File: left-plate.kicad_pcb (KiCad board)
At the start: 2 copper layers, 155.6 x 97.3 mm, 26 parts

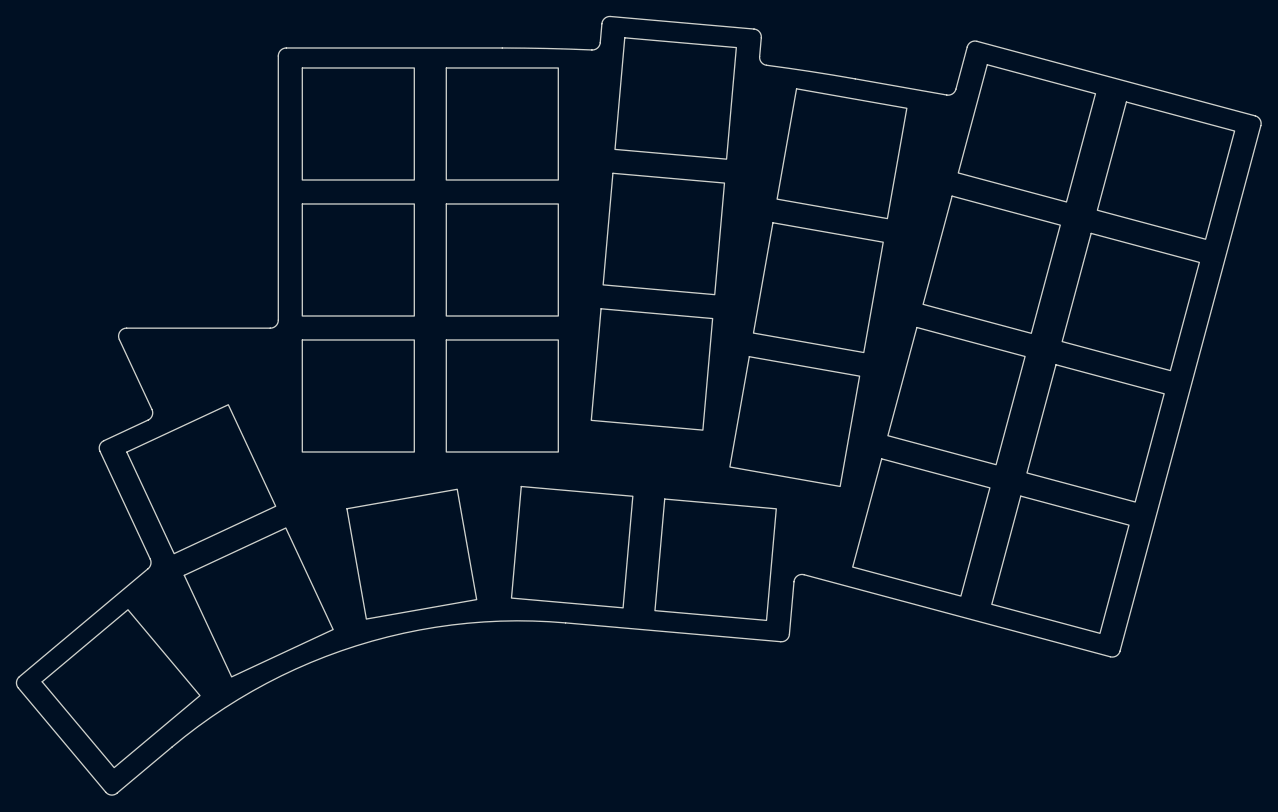
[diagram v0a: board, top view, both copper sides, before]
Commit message: update plates
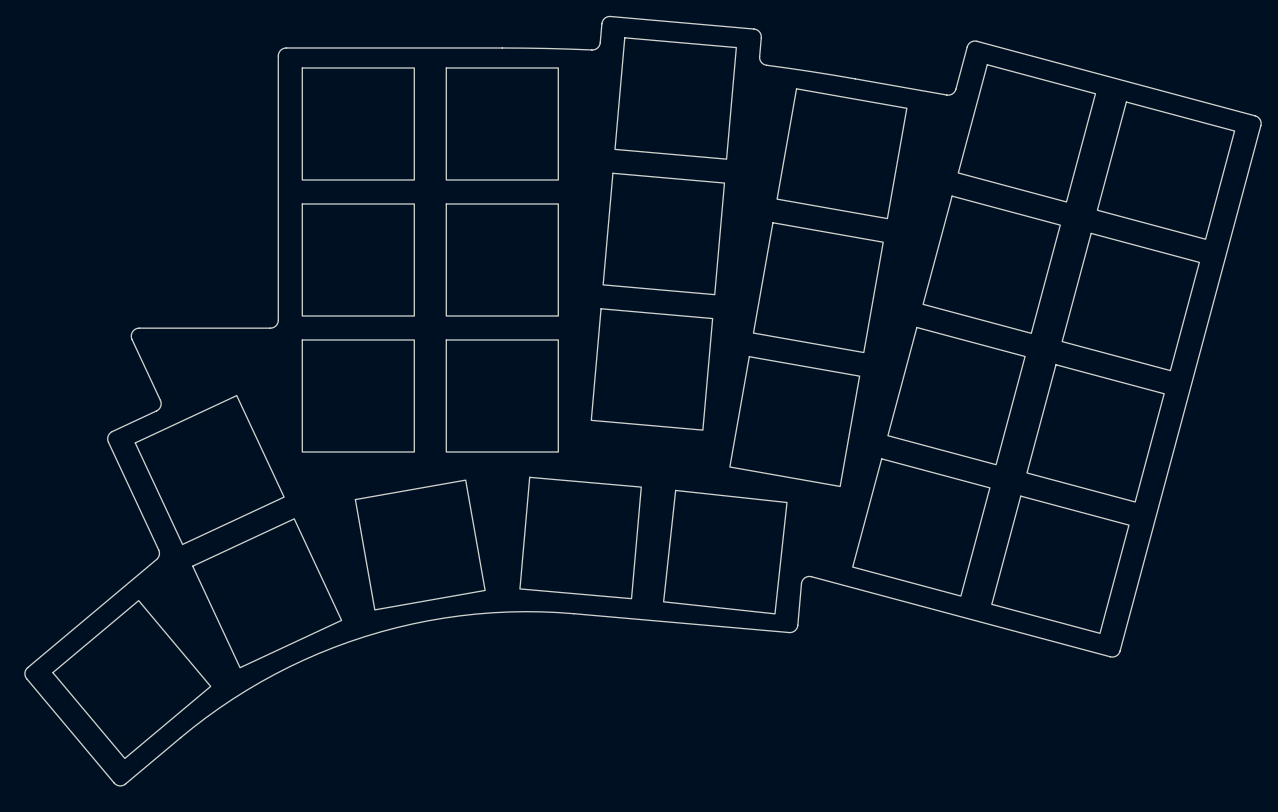
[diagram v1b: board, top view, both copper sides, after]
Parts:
- moved REF** 1.76 mm to (51.5, 128.9)
- moved REF** 1.56 mm to (107.6, 111.3)
- moved REF** 1.56 mm to (68.4, 118.2)
- moved REF** 1.56 mm to (61.2, 102.8)
- moved REF** 1.56 mm to (87.5, 112.1)
- moved REF** 1.54 mm to (125.7, 113.0), turned to -6.171 degrees
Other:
- board size 155.6 x 97.3 mm -> 154.5 x 96.2 mm
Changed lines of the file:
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@@
   )
   (footprint "keyboard:KeyHole" (layer "F.Cu")
-    (at 60.145785 103.89932 25)
+    (at 61.201051 102.753693 25)
     (fp_text reference "REF**" (at 0 0 25 unlocked) (layer "F.Fab") hide
       (effects (font (size 1 1) (thickness 0.1)))
@@
   )
   (footprint "keyboard:KeyHole" (layer "F.Cu")
-    (at 106.512436 112.397684 -5)
+    (at 107.567703 111.252057 -5)
     (fp_text reference "REF**" (at 0 0 -5 unlocked) (layer "F.Fab") hide
       (effects (font (size 1 1) (thickness 0.1)))
@@
   )
   (footprint "keyboard:KeyHole" (layer "F.Cu")
-    (at 124.443941 113.966487 -5)
-    (fp_text reference "REF**" (at 0 0 -5 unlocked) (layer "F.Fab") hide
-      (effects (font (size 1 1) (thickness 0.1)))
-    )
-    (fp_text value "KeyHole" (at 0 2 -5 unlocked) (layer "F.Fab") hide
+    (at 125.654248 113.020897 -6.171)
+    (fp_text reference "REF**" (at 0 0 -6.171 unlocked) (layer "F.Fab") hide
+      (effects (font (size 1 1) (thickness 0.1)))
+    )
+    (fp_text value "KeyHole" (at 0 2 -6.171 unlocked) (layer "F.Fab") hide
       (effects (font (size 1 1) (thickness 0.125)))
     )
@@
   )
   (footprint "keyboard:KeyHole" (layer "F.Cu")
-    (at 67.330295 119.306552 25)
+    (at 68.385562 118.160925 25)
     (fp_text reference "REF**" (at 0 0 25 unlocked) (layer "F.Fab") hide
       (effects (font (size 1 1) (thickness 0.1)))
@@
   )
   (footprint "keyboard:KeyHole" (layer "F.Cu")
-    (at 86.466581 113.272904 10)
+    (at 87.521848 112.127278 10)
     (fp_text reference "REF**" (at 0 0 10 unlocked) (layer "F.Fab") hide
       (effects (font (size 1 1) (thickness 0.1)))
@@
   )
   (footprint "keyboard:KeyHole" (layer "F.Cu")
-    (at 50.124844 130.087443 40)
+    (at 51.462952 128.941816 40)
     (fp_text reference "REF**" (at 0 0 40 unlocked) (layer "F.Fab") hide
       (effects (font (size 1 1) (thickness 0.1)))
@@
     (fp_rect (start -7 -7) (end 7 7) (layer "Edge.Cuts") (stroke (width 0.12) (type default)) (fill none))
   )
-  (gr_arc (start 97.78 50.000001) (mid 103.382237 50.06179) (end 108.981748 50.247128) (layer "Edge.Cuts") (width 0.12))
+  (gr_arc (start 57.569435 136.219239) (mid 80.612677 123.577284) (end 106.739723 120.715907) (layer "Edge.Cuts") (width 0.12))
+  (gr_arc (start 97.78 50) (mid 103.382237 50.061789) (end 108.981748 50.247127) (layer "Edge.Cuts") (width 0.12))
   (gr_arc (start 110.022044 49.335256) (mid 109.685013 50.000098) (end 108.981748 50.247126) (layer "Edge.Cuts") (width 0.12))
-  (gr_line (start 47.490452 100.421886) (end 53.772947 113.894741) (layer "Edge.Cuts") (width 0.12))
+  (gr_line (start 48.545718 99.276259) (end 54.828214 112.749115) (layer "Edge.Cuts") (width 0.12))
   (gr_line (start 69.78 51) (end 69.78 84.02) (layer "Edge.Cuts") (width 0.12))
-  (gr_arc (start 134.24122 116.720205) (mid 134.663841 115.988213) (end 135.496234 115.841441) (layer "Edge.Cuts") (width 0.12))
   (gr_line (start 110.228748 46.972619) (end 110.022044 49.335256) (layer "Edge.Cuts") (width 0.12))
-  (gr_arc (start 53.772946 113.894741) (mid 53.842935 114.533799) (end 53.509427 115.083404) (layer "Edge.Cuts") (width 0.12))
-  (gr_line (start 53.509427 115.083404) (end 37.406804 128.59511) (layer "Edge.Cuts") (width 0.12))
+  (gr_arc (start 55.041575 94.040436) (mid 55.07496 94.805074) (end 54.557885 95.369362) (layer "Edge.Cuts") (width 0.12))
+  (gr_line (start 54.564694 113.937777) (end 38.46207 127.449483) (layer "Edge.Cuts") (width 0.12))
   (gr_line (start 141.886567 53.858826) (end 153.339152 55.878225) (layer "Edge.Cuts") (width 0.12))
   (gr_arc (start 69.78 84.02) (mid 69.487107 84.727107) (end 68.78 85.02) (layer "Edge.Cuts") (width 0.12))
   (gr_arc (start 129.243603 47.632383) (mid 129.922491 47.98579) (end 130.152642 48.715734) (layer "Edge.Cuts") (width 0.12))
-  (gr_line (start 134.24122 116.720205) (end 133.665064 123.305699) (layer "Edge.Cuts") (width 0.12))
+  (gr_line (start 135.17438 116.970262) (end 134.720331 122.160072) (layer "Edge.Cuts") (width 0.12))
   (gr_line (start 174.998839 125.390856) (end 192.598534 59.7079) (layer "Edge.Cuts") (width 0.12))
-  (gr_line (start 53.502619 96.514989) (end 47.974141 99.09296) (layer "Edge.Cuts") (width 0.12))
-  (gr_line (start 173.774094 126.097963) (end 135.496234 115.841441) (layer "Edge.Cuts") (width 0.12))
-  (gr_arc (start 53.986309 95.186063) (mid 54.019693 95.950701) (end 53.502619 96.514989) (layer "Edge.Cuts") (width 0.12))
+  (gr_line (start 54.557885 95.369362) (end 49.029408 97.947333) (layer "Edge.Cuts") (width 0.12))
+  (gr_line (start 173.774094 126.097963) (end 136.429395 116.091481) (layer "Edge.Cuts") (width 0.12))
+  (gr_arc (start 135.17438 116.970262) (mid 135.596995 116.238258) (end 136.429395 116.091481) (layer "Edge.Cuts") (width 0.12))
   (gr_line (start 70.78 50) (end 97.78 50) (layer "Edge.Cuts") (width 0.12))
-  (gr_line (start 132.581714 124.214738) (end 105.684457 121.861533) (layer "Edge.Cuts") (width 0.12))
+  (gr_line (start 133.63698 123.069111) (end 106.739723 120.715906) (layer "Edge.Cuts") (width 0.12))
   (gr_line (start 191.891427 58.483155) (end 157.118097 49.16567) (layer "Edge.Cuts") (width 0.12))
   (gr_arc (start 174.998839 125.390856) (mid 174.532913 125.998062) (end 173.774094 126.097963) (layer "Edge.Cuts") (width 0.12))
-  (gr_arc (start 133.665064 123.305699) (mid 133.311657 123.984588) (end 132.581714 124.214738) (layer "Edge.Cuts") (width 0.12))
   (gr_arc (start 110.228748 46.972619) (mid 110.582155 46.293731) (end 111.312099 46.06358) (layer "Edge.Cuts") (width 0.12))
   (gr_line (start 129.945938 51.07837) (end 130.152642 48.715734) (layer "Edge.Cuts") (width 0.12))
-  (gr_arc (start 47.490452 100.421886) (mid 47.457067 99.657248) (end 47.974141 99.09296) (layer "Edge.Cuts") (width 0.12))
-  (gr_line (start 49.619768 143.149954) (end 56.514168 137.364866) (layer "Edge.Cuts") (width 0.12))
+  (gr_line (start 50.675035 142.004327) (end 57.569435 136.219239) (layer "Edge.Cuts") (width 0.12))
+  (gr_arc (start 50.675034 142.004326) (mid 49.945092 142.234476) (end 49.266203 141.88107) (layer "Edge.Cuts") (width 0.12))
   (gr_line (start 155.893352 49.872776) (end 154.478726 55.152236) (layer "Edge.Cuts") (width 0.12))
-  (gr_line (start 48.210936 143.026697) (end 37.283547 130.003942) (layer "Edge.Cuts") (width 0.12))
+  (gr_arc (start 54.828213 112.749115) (mid 54.898201 113.388172) (end 54.564693 113.937776) (layer "Edge.Cuts") (width 0.12))
+  (gr_line (start 49.266203 141.88107) (end 38.338813 128.858315) (layer "Edge.Cuts") (width 0.12))
   (gr_arc (start 130.812085 52.157035) (mid 130.162398 51.791639) (end 129.945937 51.07837) (layer "Edge.Cuts") (width 0.12))
-  (gr_arc (start 49.619768 143.149954) (mid 48.889825 143.380104) (end 48.210937 143.026696) (layer "Edge.Cuts") (width 0.12))
-  (gr_line (start 53.986308 95.186063) (end 49.909173 86.442618) (layer "Edge.Cuts") (width 0.12))
+  (gr_arc (start 48.545718 99.276259) (mid 48.512333 98.511621) (end 49.029408 97.947333) (layer "Edge.Cuts") (width 0.12))
+  (gr_arc (start 51.498654 86.442618) (mid 51.561571 85.4827) (end 52.404962 85.02) (layer "Edge.Cuts") (width 0.12))
+  (gr_line (start 55.041575 94.040436) (end 51.498654 86.442618) (layer "Edge.Cuts") (width 0.12))
   (gr_arc (start 130.812085 52.157035) (mid 136.358711 52.946858) (end 141.886567 53.858826) (layer "Edge.Cuts") (width 0.12))
-  (gr_line (start 50.815481 85.02) (end 68.78 85.02) (layer "Edge.Cuts") (width 0.12))
+  (gr_arc (start 134.720331 122.160072) (mid 134.366924 122.838961) (end 133.63698 123.069112) (layer "Edge.Cuts") (width 0.12))
+  (gr_line (start 52.404962 85.02) (end 68.78 85.02) (layer "Edge.Cuts") (width 0.12))
   (gr_arc (start 191.891427 58.483155) (mid 192.498633 58.949081) (end 192.598534 59.7079) (layer "Edge.Cuts") (width 0.12))
   (gr_arc (start 69.78 51) (mid 70.072893 50.292893) (end 70.78 50) (layer "Edge.Cuts") (width 0.12))
@@
   (gr_arc (start 155.893352 49.872776) (mid 156.359278 49.26557) (end 157.118097 49.16567) (layer "Edge.Cuts") (width 0.12))
   (gr_arc (start 154.478726 55.152236) (mid 154.050098 55.736805) (end 153.339152 55.878225) (layer "Edge.Cuts") (width 0.12))
-  (gr_arc (start 56.514168 137.364866) (mid 79.55741 124.72291) (end 105.684457 121.861534) (layer "Edge.Cuts") (width 0.12))
-  (gr_arc (start 49.909173 86.442618) (mid 49.97209 85.4827) (end 50.815481 85.02) (layer "Edge.Cuts") (width 0.12))
-  (gr_arc (start 37.283548 130.003941) (mid 37.053398 129.273999) (end 37.406804 128.59511) (layer "Edge.Cuts") (width 0.12))
+  (gr_arc (start 38.338814 128.858315) (mid 38.108663 128.128372) (end 38.46207 127.449483) (layer "Edge.Cuts") (width 0.12))
 )
